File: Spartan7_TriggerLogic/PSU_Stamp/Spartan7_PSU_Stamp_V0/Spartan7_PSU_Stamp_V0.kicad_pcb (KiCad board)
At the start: 4 copper layers, 54.8 x 55.8 mm, 37 parts, among them J1 USB4125-GF-A, U1 LT3081EDF-TRPBF, U2 LT3081EDF-TRPBF, U3 TPS7A8801RTJT, U4 TPS7A8801RTJT

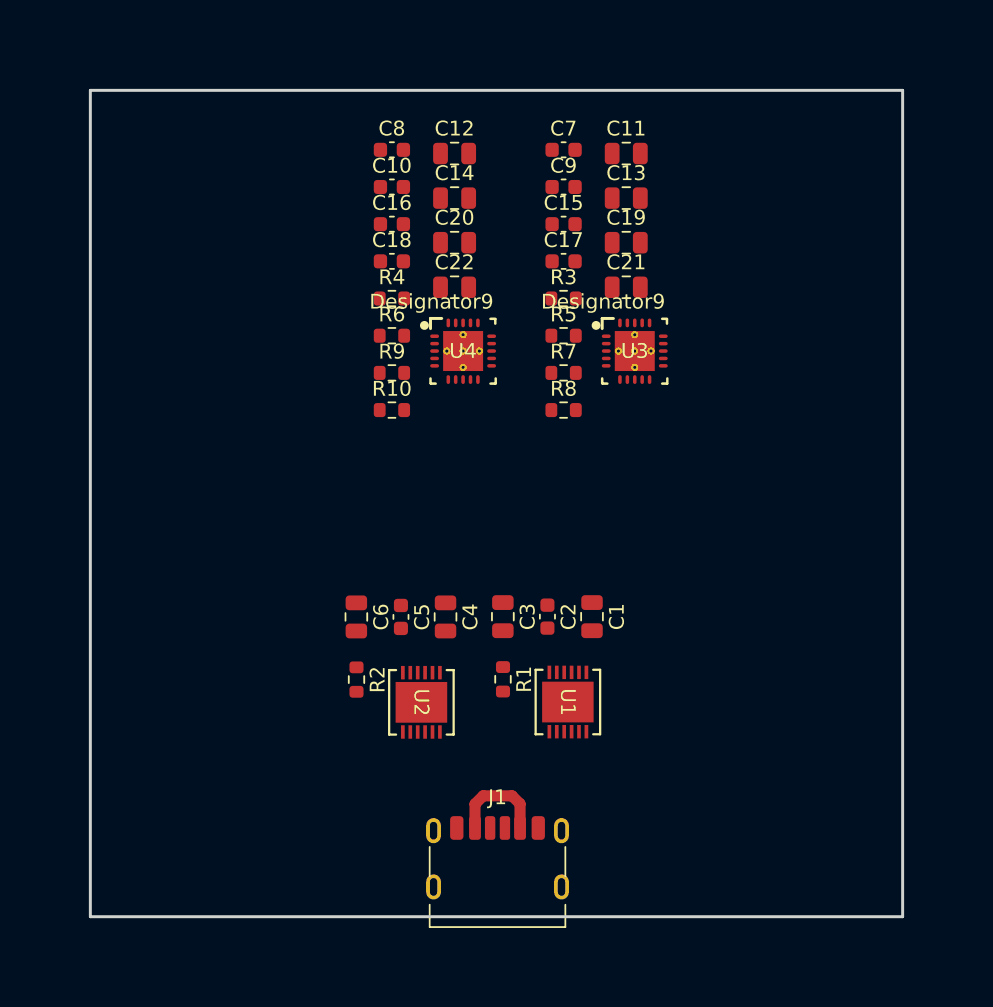
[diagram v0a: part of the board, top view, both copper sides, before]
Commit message: .
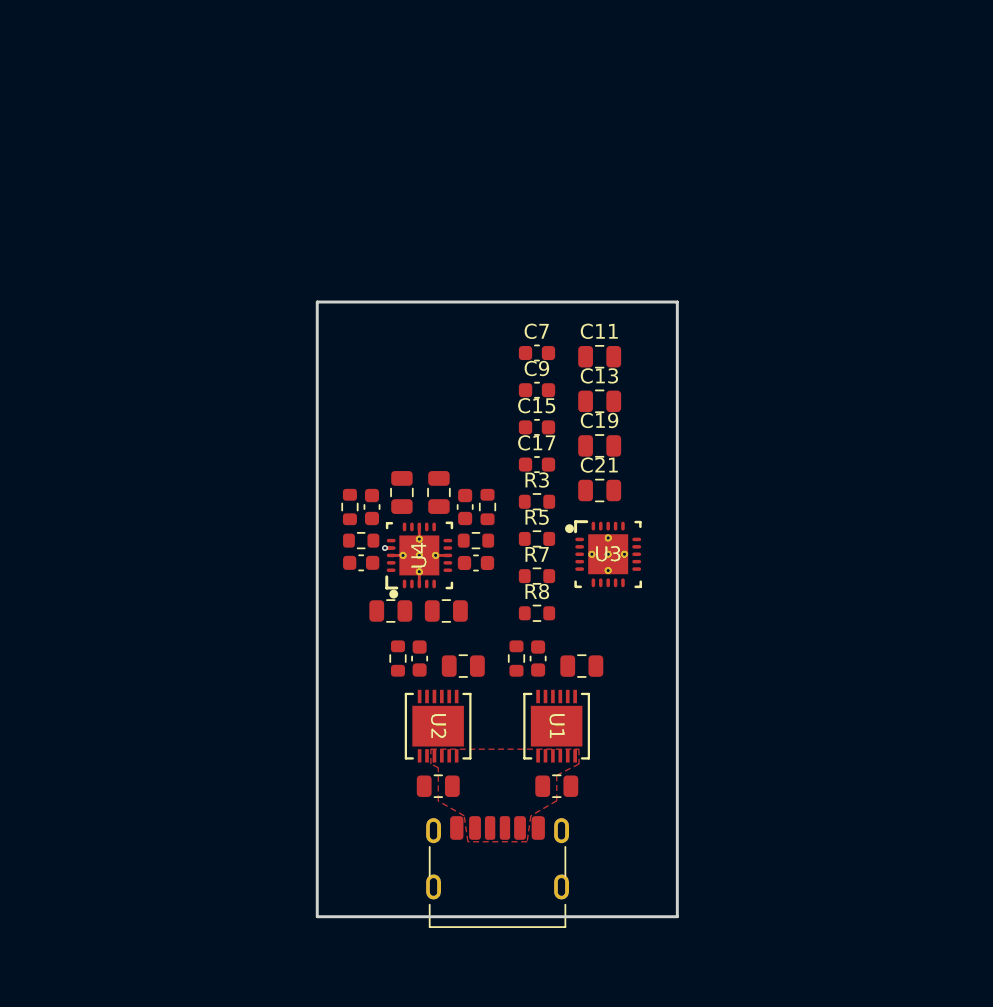
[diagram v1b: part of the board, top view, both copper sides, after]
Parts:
- moved C12 31.2 mm to (128.9, 91.9), turned to 180 degrees
- moved C8 28.0 mm to (126.9, 88.7), turned to 180 degrees
- moved C14 27.9 mm to (132.6, 91.9)
- moved C10 26.0 mm to (134.6, 88.7)
- moved C16 19.1 mm to (127.6, 84.9), turned to -90 degrees
- moved C18 17.3 mm to (133.9, 84.9), turned to -90 degrees
- moved C20 16.9 mm to (132.1, 83.9), turned to 90 degrees
- moved R4 15.5 mm to (135.4, 84.9), turned to -90 degrees
- moved R6 15.0 mm to (134.6, 87.2)
- moved C22 14.3 mm to (129.6, 83.9), turned to 90 degrees
- moved U4 14.1 mm to (130.8, 88.2), turned to 90 degrees
- moved C15 13.8 mm to (138.8, 79.5)
- moved C7 13.8 mm to (138.8, 74.5)
- moved R3 13.8 mm to (138.8, 84.5)
- moved R5 13.8 mm to (138.8, 87.0)
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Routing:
- net +5V: track 6.74 -> 0.00 mm
- net GND: track 0.00 -> 3.28 mm
- net /3.6V-3.3V/EN_2: track 0.00 -> 0.42 mm, vias 0 -> 1
- added copper zone on F.Cu, net +5V
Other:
- board size 54.8 x 55.8 mm -> 24.3 x 41.5 mm
